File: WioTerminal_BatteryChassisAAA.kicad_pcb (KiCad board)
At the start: 2 copper layers, 67.5 x 52.6 mm, 0 parts

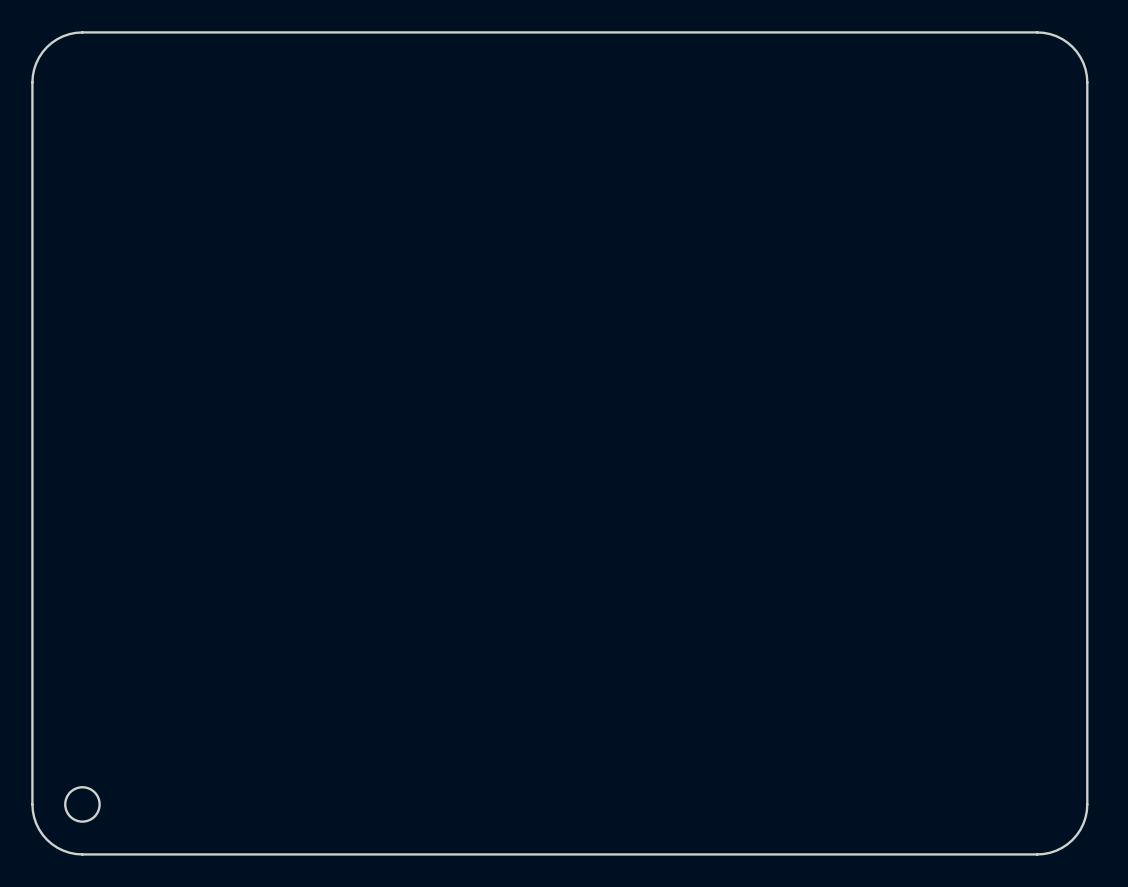
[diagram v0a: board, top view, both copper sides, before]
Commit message: Revision A
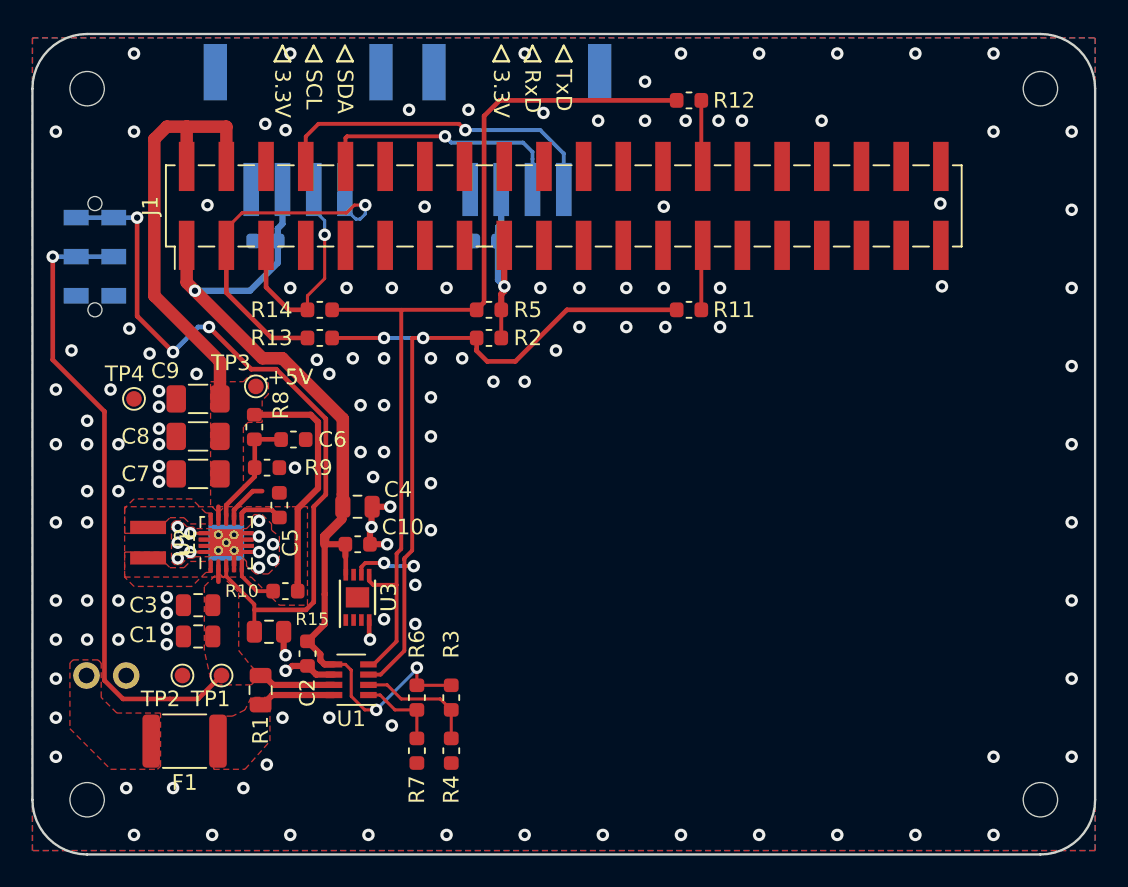
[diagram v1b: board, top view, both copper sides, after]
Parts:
- added C1: 10u, Capacitor_SMD:C_0805_2012Metric, F.Cu at (10.6, -13.9)
- added C10: 100n, Capacitor_SMD:C_0603_1608Metric, F.Cu at (20.8, -19.9)
- added C12: 1u, Capacitor_SMD:C_0603_1608Metric, B.Cu at (29.0, -39.2)
- added C13: 1u, Capacitor_SMD:C_0603_1608Metric, B.Cu at (14.9, -39.2)
- added C2: 100n, Capacitor_SMD:C_0603_1608Metric, F.Cu at (17.6, -12.8)
- added C3: 10u, Capacitor_SMD:C_0805_2012Metric, F.Cu at (10.6, -15.9)
- added C4: 10u, Capacitor_SMD:C_0805_2012Metric, F.Cu at (20.8, -22.2)
- added C5: 100n, Capacitor_SMD:C_0603_1608Metric, F.Cu at (15.8, -22.4)
- added C6: 10p, Capacitor_SMD:C_0603_1608Metric, F.Cu at (16.7, -26.6)
- added C7: 22u, Capacitor_SMD:C_1206_3216Metric, F.Cu at (10.6, -24.4)
- added C8: 22u, Capacitor_SMD:C_1206_3216Metric, F.Cu at (10.6, -26.8)
- added C9: 22u, Capacitor_SMD:C_1206_3216Metric, F.Cu at (10.6, -29.1)
- added F1: 1A, Fuse:Fuse_1812_4532Metric, F.Cu at (9.74, -7.25)
- added J1: Raspberry_Pi_2_3, Connector_PinHeader_2.54mm:PinHeader_2x20_P2.54mm_Vertical_SMD, F.Cu at (34.0, -41.5)
- added J2: Ext. BAT, local:PinHeader_1x02_P2.54mm_Horizontal, B.Cu at (3.46, -11.4)
- added J3: GROVE, local:PHS-4AW, B.Cu at (31.0, -44.2)
- added J4: GROVE, local:PHS-4AW, B.Cu at (17.0, -44.2)
- added L1: 1u, 2.5A, local:74438323010, F.Cu at (7.40, -19.9)
- added LOGO1: Logo_Open_Hardware_Small, local:logo, B.Cu at (31.8, -5.25)
- added MH1: Corner, local:MountingHole_2.2mm_M2_DIN965_Mask, F.Cu at (3.50, -3.50)
- added MH2: Corner, local:MountingHole_2.2mm_M2_DIN965_Mask, F.Cu at (64.5, -3.50)
- added MH3: Corner, local:MountingHole_2.2mm_M2_DIN965_Mask, F.Cu at (64.5, -49.0)
- added MH4: Corner, local:MountingHole_2.2mm_M2_DIN965_Mask, F.Cu at (3.50, -49.0)
- added R1: 0.04, Resistor_SMD:R_0805_2012Metric, F.Cu at (14.6, -10.5)
- added R10: 1M, Resistor_SMD:R_0603_1608Metric, F.Cu at (16.2, -16.9)
- added R11: 0, Resistor_SMD:R_0603_1608Metric, F.Cu at (42.0, -34.9)
- added R12: 0, Resistor_SMD:R_0603_1608Metric, F.Cu at (42.0, -48.2)
- added R13: DNP, Resistor_SMD:R_0603_1608Metric, F.Cu at (18.4, -33.0)
- added R14: DNP, Resistor_SMD:R_0603_1608Metric, F.Cu at (18.4, -34.9)
- added R15: 100k, Resistor_SMD:R_0805_2012Metric, F.Cu at (15.1, -14.2)
- added R2: 4.7k, Resistor_SMD:R_0603_1608Metric, F.Cu at (29.2, -33.0)
- added R3: 0, Resistor_SMD:R_0603_1608Metric, F.Cu at (26.8, -10.0)
- added R4: DNP, Resistor_SMD:R_0603_1608Metric, F.Cu at (26.8, -6.64)
- added R5: 4.7k, Resistor_SMD:R_0603_1608Metric, F.Cu at (29.2, -34.9)
- added R6: 0, Resistor_SMD:R_0603_1608Metric, F.Cu at (24.6, -10.0)
- added R7: DNP, Resistor_SMD:R_0603_1608Metric, F.Cu at (24.6, -6.64)
- added R8: 1M, Resistor_SMD:R_0603_1608Metric, F.Cu at (14.2, -27.4)
- added R9: 111k, Resistor_SMD:R_0603_1608Metric, F.Cu at (15.0, -24.8)
- added SW1: JS102011JAQN, local:JS102011JAQN, B.Cu at (4.00, -38.2)
- added TP1: BAT, TestPoint:TestPoint_Pad_D1.0mm, F.Cu at (12.1, -11.4)
- added TP2: BAT-GND, TestPoint:TestPoint_Pad_D1.0mm, F.Cu at (9.60, -11.4)
- added TP3: +5V, TestPoint:TestPoint_Pad_D1.0mm, F.Cu at (14.3, -29.9)
- added TP4: +5V-GND, TestPoint:TestPoint_Pad_D1.0mm, F.Cu at (6.50, -29.1)
- added U1: INA219, Package_TO_SOT_SMD:SOT-23-8, F.Cu at (20.4, -11.2)
- added U2: TPS63060, Package_SON:Texas_S-PWSON-N10_ThermalVias, F.Cu at (12.4, -19.9)
- added U3: ATECC608A, Package_DFN_QFN:DFN-8-1EP_3x2mm_P0.5mm_EP1.3x1.5mm, F.Cu at (20.8, -16.4)
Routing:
- net +3V3: track 0.00 -> 72.5 mm, vias 0 -> 4
- net /SCL: track 0.00 -> 60.6 mm
- net /SDA: track 0.00 -> 53.0 mm, vias 0 -> 4
- net Net-(R15-Pad2): track 0.00 -> 47.3 mm, vias 0 -> 3
- net Net-(C1-Pad1): track 0.00 -> 47.0 mm, vias 0 -> 1
- net +5V: track 0.00 -> 44.8 mm
- net /I2C1_SDA: track 0.00 -> 23.5 mm, vias 0 -> 1
- net /TXD: track 0.00 -> 21.8 mm, vias 0 -> 1
- net GND: track 0.00 -> 17.0 mm, vias 0 -> 142
- net /RXD: track 0.00 -> 16.7 mm, vias 0 -> 1
- net /I2C1_SCL: track 0.00 -> 14.4 mm, vias 0 -> 1
- net /A0: track 0.00 -> 7.79 mm
- net Net-(C6-Pad1): track 0.00 -> 7.34 mm
- net /A1: track 0.00 -> 5.32 mm
- net Net-(F1-Pad1): track 0.00 -> 4.96 mm
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- added copper zone on F.Cu, net +5V
- added copper zone on B.Cu, net GND
- added copper zone on F.Cu, net GND
- added copper zone on F.Cu, net Net-(C1-Pad1)
- added copper zone on F.Cu, net Net-(F1-Pad1)
- added copper zone on F.Cu, net Net-(F1-Pad2)
- added copper zone on F.Cu, net Net-(L1-Pad1)
- added copper zone on F.Cu, net Net-(L1-Pad2)
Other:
- board size 67.5 x 52.6 mm -> 68 x 52.5 mm
- board text added: "+5V"
- board text added: "3.3V"
- board text added: "AA/AAA Battery Chassis for Wio Terminal 2020-05-28 Rev.A by Kenta IDA (@ciniml)"
- board text added: "ON"
- board text added: "RxD"
- board text added: "SCL"
- board text added: "SDA"
- board text added: "TxD"
